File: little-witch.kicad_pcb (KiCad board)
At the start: 4 copper layers, 65 x 30 mm, 56 parts, among them J1 GCT-USB4105, J2 TMJG0803HENL, J3 Conn_ARM_SWD_TagConnect_TC203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, J4 GCT-USB4105, J5 Conn_02x20_Odd_Even, J6 BOOT0_SEL, SW1 SW_Push, U1 CH32V307RCT6, U2 MXL86110C-AQB-R, Y1 SIT8008BI-73-33N-25.000000

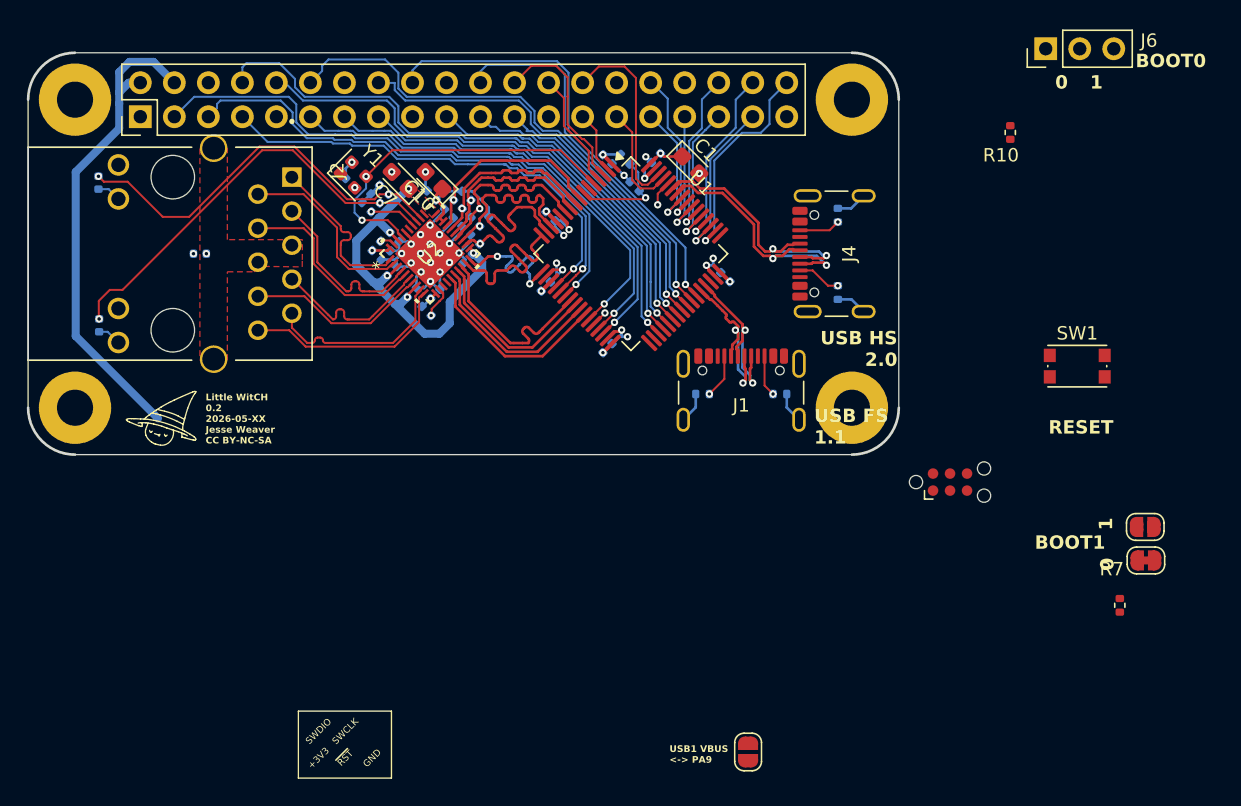
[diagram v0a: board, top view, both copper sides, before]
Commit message: Power regulation
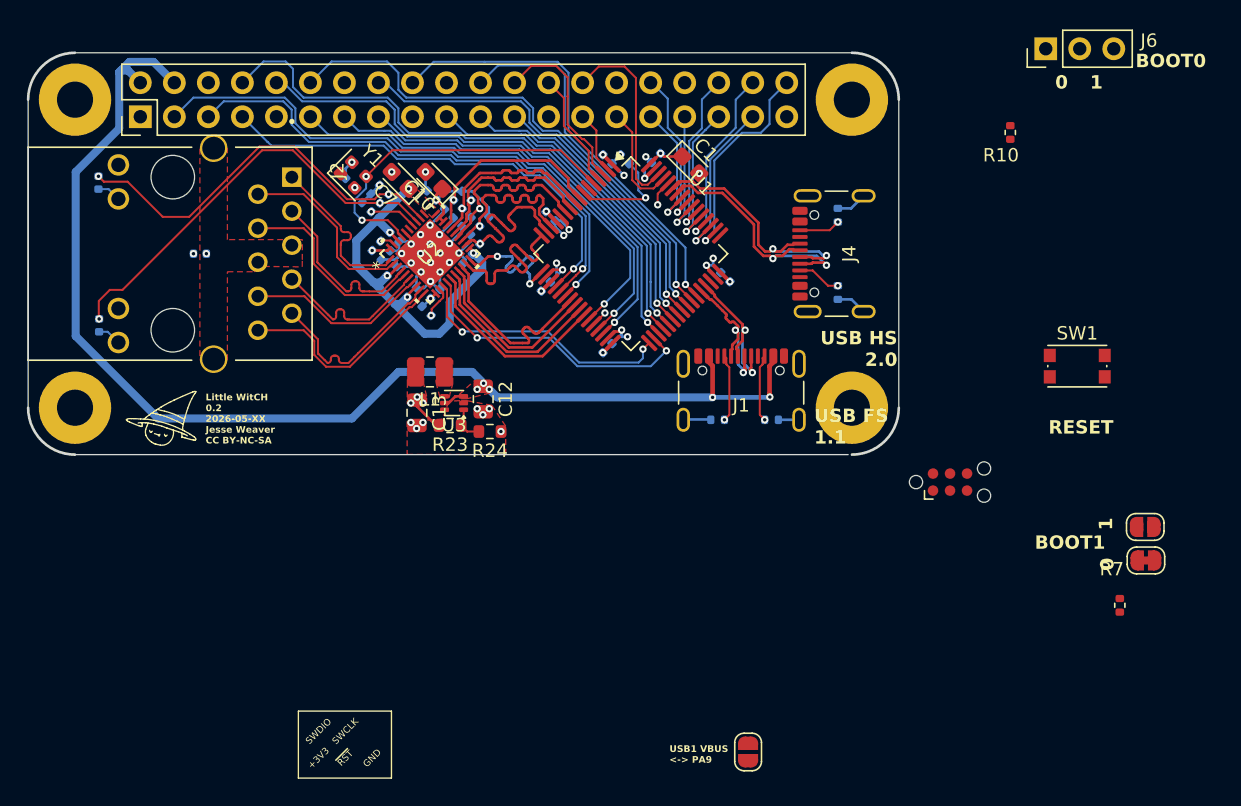
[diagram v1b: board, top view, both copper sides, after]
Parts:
- removed R1: 10k, Resistor_SMD:R_0402_1005Metric
- added C12: 4.7u, Capacitor_SMD:C_0805_2012Metric, F.Cu at (134.0, 125.9)
- added C13: 22u, Capacitor_SMD:C_0805_2012Metric, F.Cu at (129.0, 126.9)
- added L1: 1u, Inductor_SMD:L_1008_2520Metric, F.Cu at (130.0, 123.8)
- added R23: 450K ±1%, Resistor_SMD:R_0603_1608Metric, F.Cu at (131.5, 127.8)
- added R24: 100K ±1%, Resistor_SMD:R_0603_1608Metric, F.Cu at (134.5, 128.3)
- added U3: TPS62A0568PDRLR, Package_TO_SOT_SMD:SOT-563, F.Cu at (131.8, 126.2)
- moved R3 2.23 mm to (151.5, 127.4)
- moved C8 2.15 mm to (144.6, 108.0)
- moved R4 2.02 mm to (155.5, 127.4)
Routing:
- net USB1_VBUS: track 36.7 -> 92.1 mm, vias 0 -> 5
- net ETH_MDIO: track 0.00 -> 21.9 mm, vias 0 -> 2
- net ETH_MDC: track 0.00 -> 20.0 mm, vias 0 -> 2
- net Net-(U3-FB): track 0.00 -> 2.77 mm
- net Net-(J1-CC2): track 3.09 -> 5.07 mm
- net Net-(J1-CC1): track 3.29 -> 5.06 mm
- net USB1_DN: track 13.2 -> 11.5 mm
- net USB1_DP: track 13.2 -> 11.6 mm
- net +3V3: track 24.4 -> 25.8 mm, vias 11 -> 14
- net /TD4-: track 15.7 -> 16.5 mm
- net /TD4+: track 14.4 -> 15.2 mm
- net GND: track 51.9 -> 51.1 mm, vias 32 -> 40
- net /PA10: track 33.8 -> 33.2 mm
- net /PA9: track 28.4 -> 27.9 mm
- added copper zone on F.Cu, net +3V3
- added copper zone on F.Cu, net GND
- added copper zone on F.Cu, net Net-(U3-SW)
- added copper zone on F.Cu, net USB1_VBUS
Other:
- outline, holes or cut-outs redrawn
